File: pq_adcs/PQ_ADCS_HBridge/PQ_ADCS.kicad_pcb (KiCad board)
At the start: 6 copper layers, 40 x 40 mm, 62 parts, among them J1 CES-110-02-L-S, J10 Pico-Clasp_01x09, J11 Pico-Clasp_01x15, J12 CES-102-02-L-S, J2 CES-110-02-L-S, J3 CES-110-02-L-S, J4 CES-110-02-L-S, J5 Pico-Clasp_01x03, J6 Pico-Clasp_01x10, J7 Pico-Clasp_01x10, J8 Pico-Clasp_01x10, J9 Pico-Clasp_01x10, U1 LPV542, U2 LPV542, U3 LPV542, U4 IIM-42652, U5 DRV8214RTER, U6 TMUX1108RSVR, U7 MMC5983MA, U8 DRV8214RTER, U9 DRV8214RTER

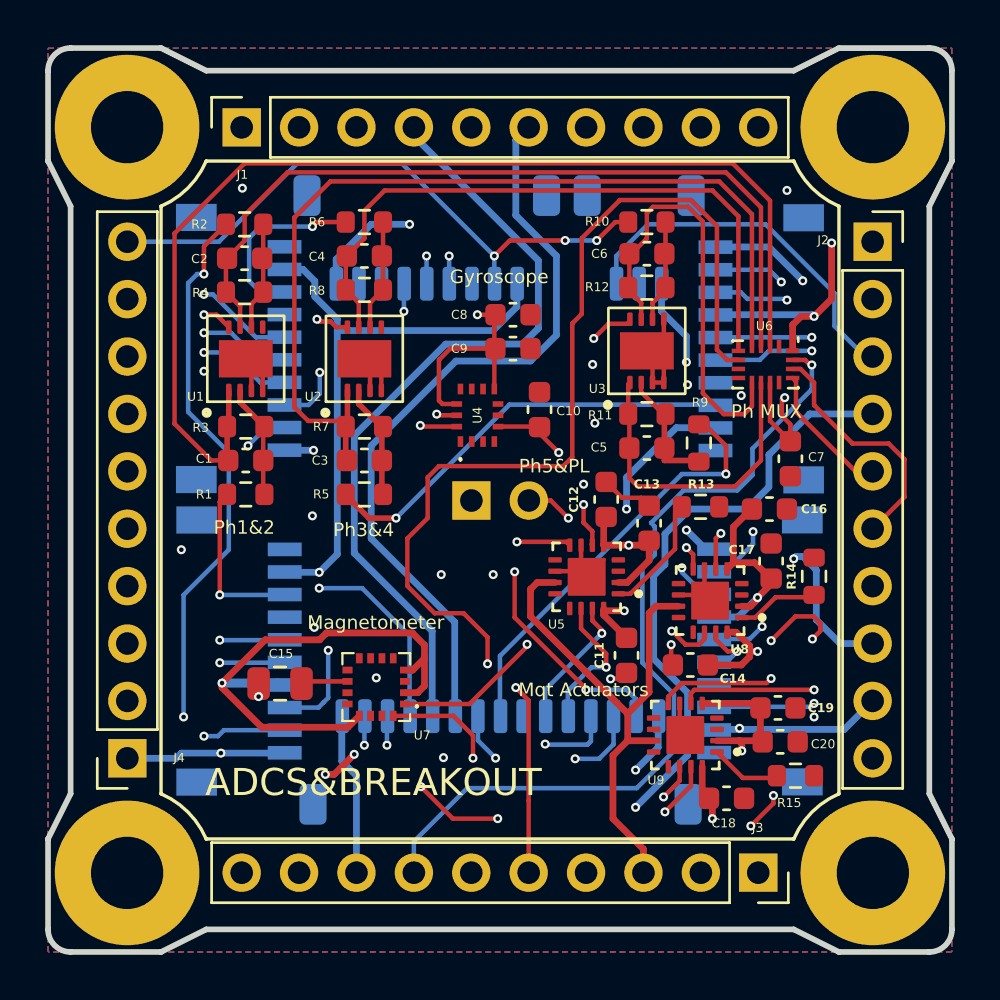
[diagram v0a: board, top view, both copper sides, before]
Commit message: Revision done
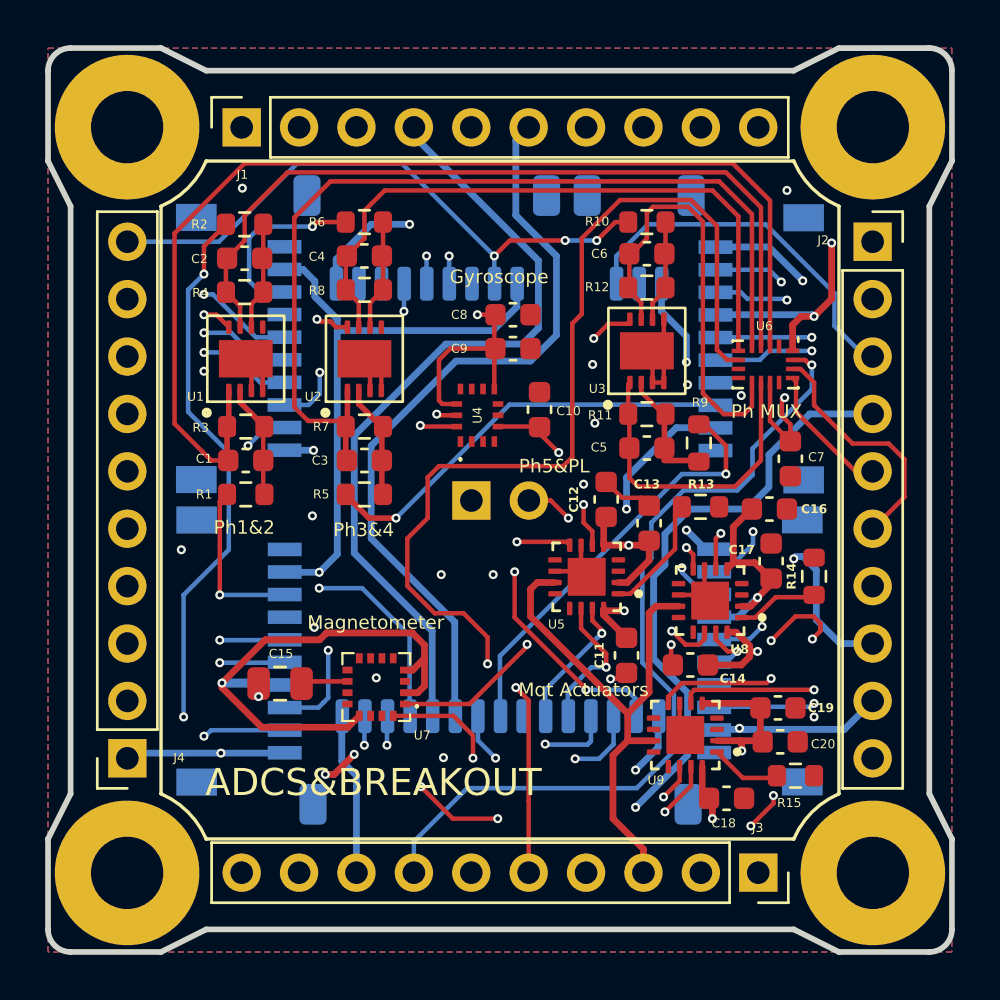
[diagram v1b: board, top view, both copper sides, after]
